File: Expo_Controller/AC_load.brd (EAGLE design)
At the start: 80 x 46 mm, 13 parts

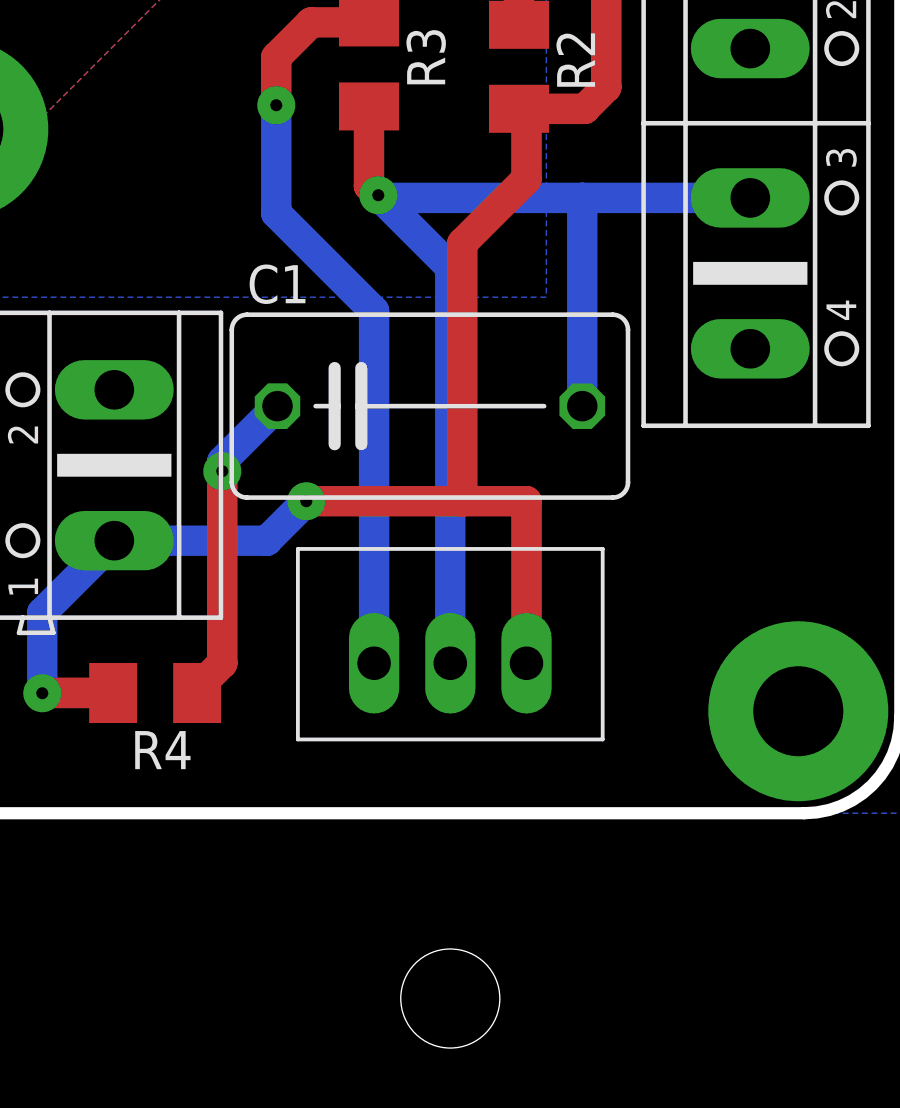
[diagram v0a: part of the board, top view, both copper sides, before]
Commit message: BugFix
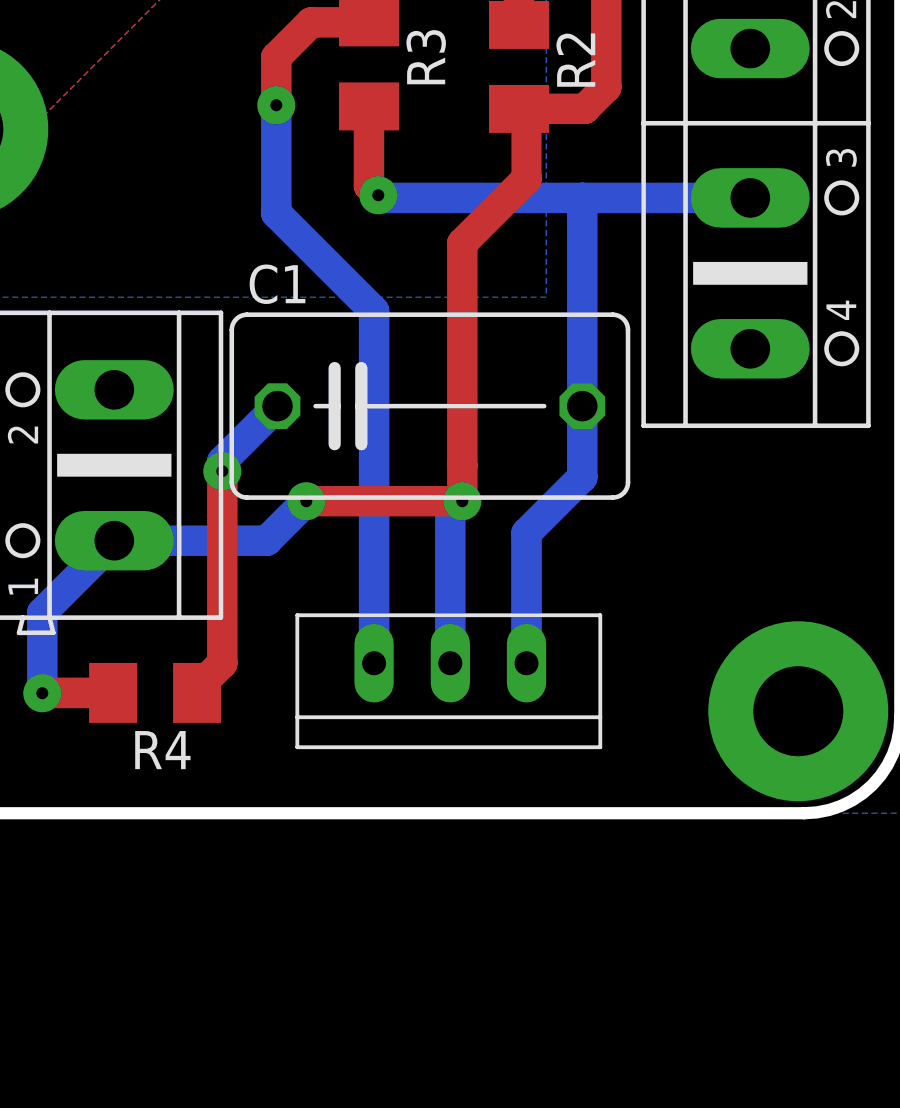
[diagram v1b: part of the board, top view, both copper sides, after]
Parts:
- U$2: device Semistors:TO220 -> Semistors:TO220NORM
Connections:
- net N$2: now also U$2.MT1; no longer U$2.IN2
- net N$4: now also U$2.GATE; no longer U$2.CONTROL
- net V+: now also U$2.MT2; no longer U$2.IN1
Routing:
- net N$2: track 39.1 -> 31.8 mm
- net V+: track 55.5 -> 53.5 mm, vias 3 -> 4
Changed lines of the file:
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@@
 <?xml version="1.0" encoding="utf-8"?>
 <!DOCTYPE eagle SYSTEM "eagle.dtd">
-<eagle version="7.1.0">
+<eagle version="6.5.0">
 <drawing>
 <settings>
@@
 <pass name="Default">
 <param name="RoutingGrid" value="50mil"/>
-<param name="AutoGrid" value="1"/>
-<param name="Efforts" value="0"/>
-<param name="TopRouterVariant" value="1"/>
 <param name="tpViaShape" value="round"/>
 <param name="PrefDir.1" value="|"/>
@@
 <attribute name="OC_FARNELL" value="unknown" x="53.8" y="34.6" size="1.778" layer="27" rot="R270" display="off"/>
 </element>
-<element name="U$2" library="Semistors" package="TO220" value="BTB16" x="65" y="5" rot="R180"/>
+<element name="U$2" library="Semistors" package="TO220NORM" value="BTB16" x="65" y="5" rot="R180"/>
 <element name="LED1" library="led" package="SML1206" value="" x="3.4" y="9.6" rot="R90"/>
 <element name="R5" library="rcl" package="M1206" value="" x="3.4" y="15.6" rot="R90"/>
@@
 <contactref element="R4" pad="2"/>
 <contactref element="X2" pad="1"/>
-<contactref element="U$2" pad="IN1"/>
+<contactref element="U$2" pad="MT2"/>
 <wire x1="75" y1="30.5184" x2="71.9184" y2="30.5184" width="1.016" layer="16"/>
 <wire x1="71.9184" y1="30.5184" x2="70.2" y2="28.8" width="1.016" layer="16"/>
@@
 <wire x1="70.2" y1="24.2" x2="69.48" y2="23.48" width="1.016" layer="1"/>
 <wire x1="69.48" y1="23.48" x2="67.29" y2="23.48" width="1.016" layer="1"/>
-<wire x1="67.54" y1="5" x2="67.54" y2="10.4" width="1.016" layer="1"/>
 <wire x1="67.54" y1="23.23" x2="67.29" y2="23.48" width="1.016" layer="1"/>
 <wire x1="53.8" y1="9.0854" x2="58.8854" y2="9.0854" width="1.016" layer="16"/>
@@
 <via x="60.2" y="10.4" extent="1-16" drill="0.4" diameter="1.27"/>
 <wire x1="60.2" y1="10.4" x2="65.4" y2="10.4" width="1.016" layer="1"/>
-<wire x1="65.4" y1="10.4" x2="67.54" y2="10.4" width="1.016" layer="1"/>
 <wire x1="53.76" y1="4.01" x2="51.41" y2="4.01" width="1.016" layer="1"/>
 <wire x1="51.41" y1="4.01" x2="51.4" y2="4" width="1.016" layer="1"/>
@@
 <wire x1="67.54" y1="23.23" x2="67.54" y2="21.14" width="1.016" layer="1"/>
 <wire x1="67.54" y1="21.14" x2="65.4" y2="19" width="1.016" layer="1"/>
-<wire x1="65.4" y1="19" x2="65.4" y2="10.4" width="1.016" layer="1"/>
+<wire x1="65.4" y1="19" x2="65.4" y2="11.6" width="1.016" layer="1"/>
+<wire x1="65" y1="5" x2="65" y2="10" width="1.016" layer="16"/>
+<wire x1="65" y1="10" x2="65.4" y2="10.4" width="1.016" layer="16"/>
+<via x="65.4" y="10.4" extent="1-16" drill="0.4" diameter="1.27"/>
+<wire x1="65.4" y1="10.4" x2="65.4" y2="11.6" width="1.016" layer="1"/>
 </signal>
 <signal name="PE">
@@
 <contactref element="C1" pad="2"/>
 <contactref element="X1" pad="3"/>
-<contactref element="U$2" pad="IN2"/>
+<contactref element="U$2" pad="MT1"/>
 <wire x1="75" y1="20.5108" x2="69.4" y2="20.5108" width="1.016" layer="16"/>
 <wire x1="69.4" y1="20.5108" x2="62.6892" y2="20.5108" width="1.016" layer="16"/>
@@
 <wire x1="62.6" y1="20.6" x2="62.29" y2="20.91" width="1.016" layer="1"/>
 <wire x1="62.29" y1="20.91" x2="62.29" y2="23.56" width="1.016" layer="1"/>
-<wire x1="65" y1="5" x2="65" y2="18.2" width="1.016" layer="16"/>
-<wire x1="65" y1="18.2" x2="62.6" y2="20.6" width="1.016" layer="16"/>
 <wire x1="69.4" y1="13.57" x2="69.4" y2="20.5108" width="1.016" layer="16"/>
+<wire x1="67.54" y1="5" x2="67.54" y2="9.34" width="1.016" layer="16"/>
+<wire x1="67.54" y1="9.34" x2="69.4" y2="11.2" width="1.016" layer="16"/>
+<wire x1="69.4" y1="11.2" x2="69.4" y2="13.57" width="1.016" layer="16"/>
 </signal>
 <signal name="N$4">
 <contactref element="U$1" pad="4"/>
 <contactref element="R3" pad="1"/>
-<contactref element="U$2" pad="CONTROL"/>
+<contactref element="U$2" pad="GATE"/>
 <wire x1="62.21" y1="30.84" x2="62.21" y2="26.44" width="1.016" layer="1"/>
 <wire x1="62.21" y1="26.44" x2="62.29" y2="26.36" width="1.016" layer="1"/>
